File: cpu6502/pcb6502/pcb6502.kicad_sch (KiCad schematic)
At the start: 26 parts, among them J1 5v Power, J2 RS232, SW1 Reset, U1 6502, U2 EEPROM, U3 RAM, U4 65C22, U5 74HC00, U6 LCD (HD44780), U7 W65C51NxP, U8 MAX232, X1 1MHz, Y1 Crystal

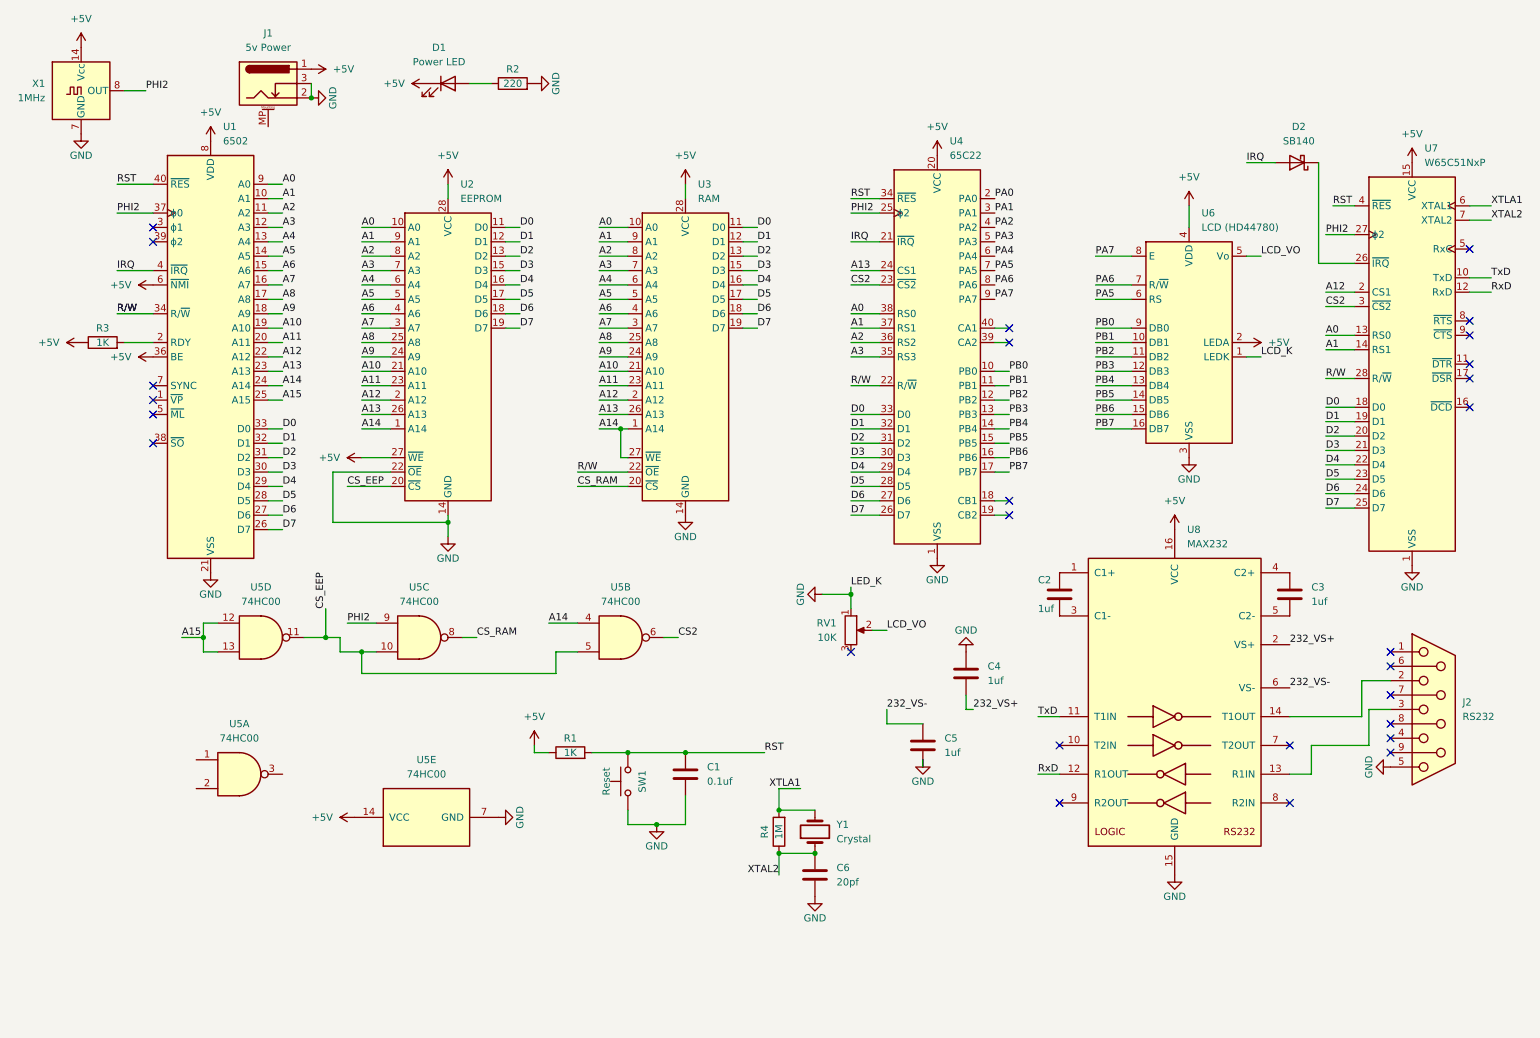
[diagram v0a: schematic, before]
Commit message: routed PCB!
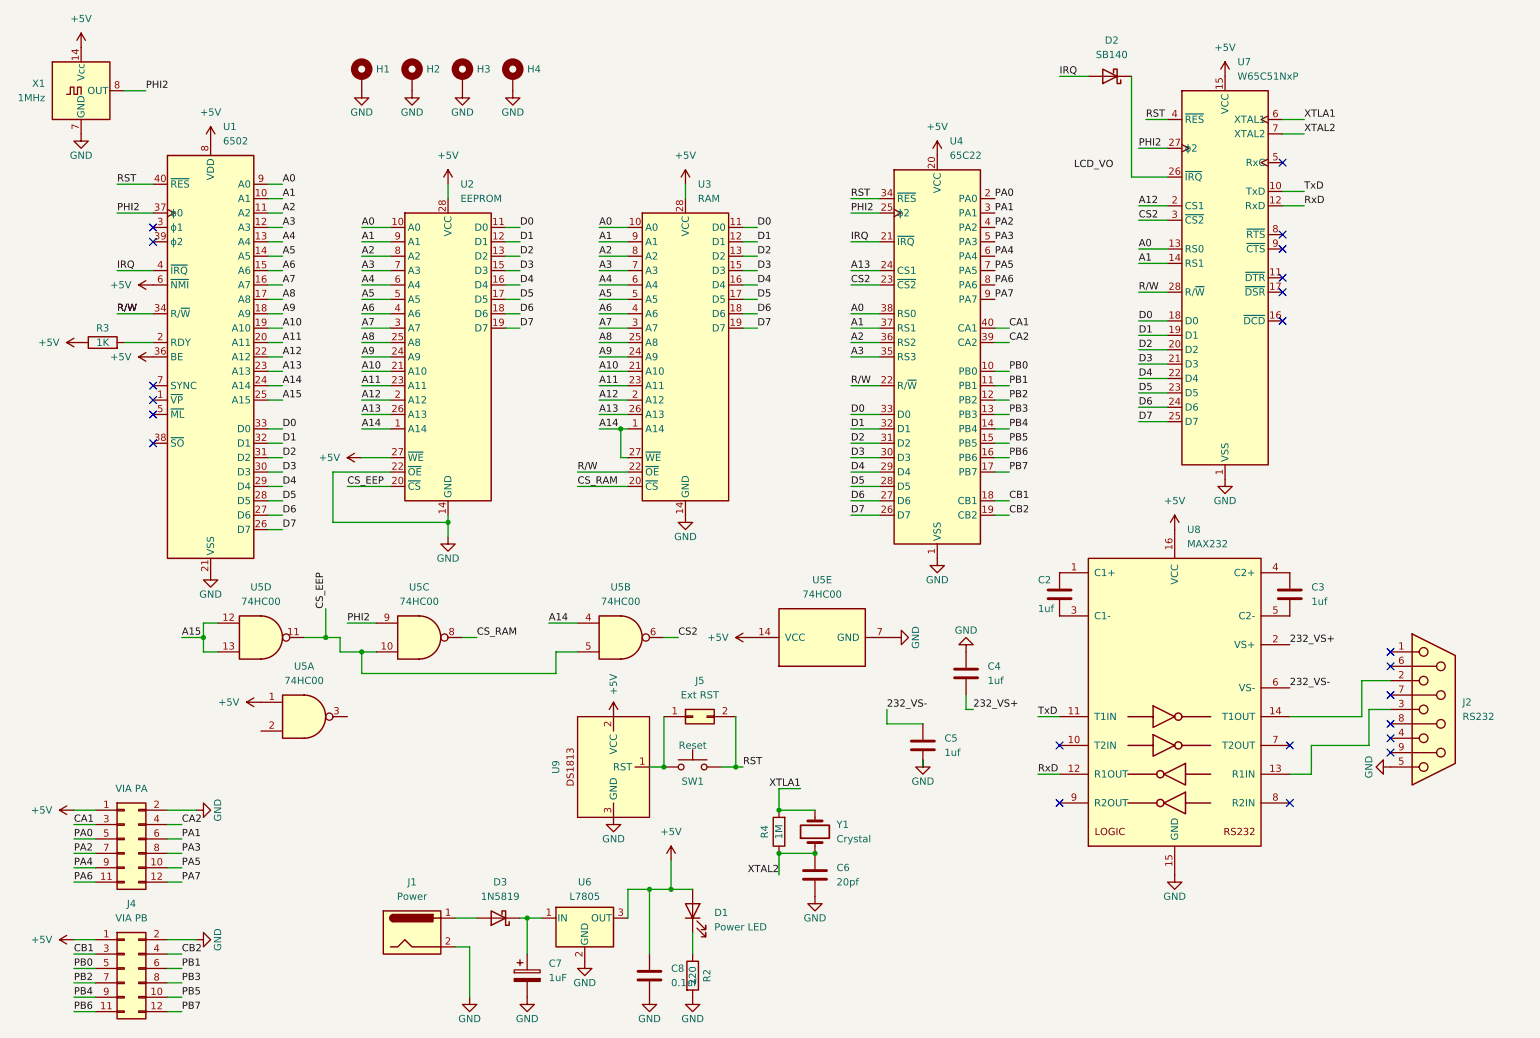
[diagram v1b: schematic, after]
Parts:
- removed C1: 0.1uf, Capacitor_THT:C_Disc_D3.0mm_W1.6mm_P2.50mm, symbol Device:C
- removed J1: 5v Power, Connector_BarrelJack:BarrelJack_CUI_PJ-102AH_Horizontal, symbol Connector:Barrel_Jack_Switch_MountingPin
- removed R1: 1K, Resistor_THT:R_Axial_DIN0204_L3.6mm_D1.6mm_P7.62mm_Horizontal, symbol Device:R
- removed RV1: 10K, Potentiometer_THT:Potentiometer_ACP_CA9-V10_Vertical, symbol Device:R_Potentiometer
- removed U6: LCD (HD44780), Display:WC1602A, symbol Display_Character:HY1602E
- added C7: 1uF, Capacitor_THT:CP_Radial_D5.0mm_P2.50mm, symbol Device:C_Polarized
- added C8: 0.1uf, Capacitor_THT:C_Disc_D3.0mm_W1.6mm_P2.50mm, symbol Device:C
- added D3: 1N5819, Diode_THT:D_DO-41_SOD81_P10.16mm_Horizontal, symbol Diode:1N5819
- added H1, H2, H3, H4: ~, MountingHole:MountingHole_3.2mm_M3_Pad_Via, symbol Mechanical:MountingHole_Pad
- added J1: Power, Connector_BarrelJack:BarrelJack_Horizontal, symbol Connector:Barrel_Jack
- added J3: VIA PA, Connector_PinHeader_2.54mm:PinHeader_2x06_P2.54mm_Vertical, symbol Connector_Generic:Conn_02x06_Odd_Even
- added J4: VIA PB, Connector_PinHeader_2.54mm:PinHeader_2x06_P2.54mm_Vertical, symbol Connector_Generic:Conn_02x06_Odd_Even
- added J5: Ext RST, Connector_PinHeader_2.54mm:PinHeader_2x01_P2.54mm_Vertical, symbol Connector_Generic:Conn_02x01
- added U6: L7805, Package_TO_SOT_THT:TO-220F-3_Horizontal_TabUp, symbol Regulator_Linear:L7805
- added U9: ~, Package_TO_SOT_THT:TO-92, symbol Power_Protection:DS1813
- U2: footprint Package_DIP:DIP-28_W15.24mm_Socket -> Package_DIP:DIP-28_600_ZIF_ARIES_28-526-10
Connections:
- net +5V: now also D1.2 (A), U5.1, C8.1, J3.1 (Pin_1), J4.1 (Pin_1), U6.3 (OUT), U9.2 (VCC); no longer D1.1 (K)
- net GND: now also C7.2, C8.2, H1.1, H2.1, H3.1, H4.1, J1.2, J3.2 (Pin_2), J4.2 (Pin_2), U6.2 (GND), U9.3 (GND); no longer SW1.1
- net PA0: now also J3.5 (Pin_5)
- net PA1: now also J3.6 (Pin_6)
- net PA2: now also J3.7 (Pin_7)
- net PA3: now also J3.8 (Pin_8)
- net PA4: now also J3.9 (Pin_9)
- net PA5: now also J3.10 (Pin_10)
- net PA6: now also J3.11 (Pin_11)
- net PA7: now also J3.12 (Pin_12)
- net PB0: now also J4.5 (Pin_5)
- net PB1: now also J4.6 (Pin_6)
- net PB2: now also J4.7 (Pin_7)
- net PB3: now also J4.8 (Pin_8)
- net PB4: now also J4.9 (Pin_9)
- net PB5: now also J4.10 (Pin_10)
- net PB6: now also J4.11 (Pin_11)
- net PB7: now also J4.12 (Pin_12)
- net RST: now also J5.2 (Pin_2)
- net CB1: now reaches U4.18 (CB1)
- net CB1: now also J4.3 (Pin_3)
- net CB2: now reaches U4.19 (CB2)
- net CB2: now also J4.4 (Pin_4)
- net CA2: now reaches U4.39 (CA2)
- net CA2: now also J3.4 (Pin_4)
- net CA1: now reaches U4.40 (CA1)
- net CA1: now also J3.3 (Pin_3)
- net at R2.1: now also D1.1 (K); no longer D1.2 (A)
- new net: J5.1 (Pin_1), SW1.1, U9.1 (RST)
- new net: C7.1, D3.1 (K), U6.1 (IN)
- new net: D3.2 (A), J1.1
- no-connect marks 27 -> 22
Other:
- moved on the sheet: D1, D2, R2, SW1, U5A, U5E, U7
